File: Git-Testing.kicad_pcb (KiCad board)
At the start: 2 copper layers, 6 parts, among them J1 Conn_01x02_Male, J2 Conn_01x02_Male

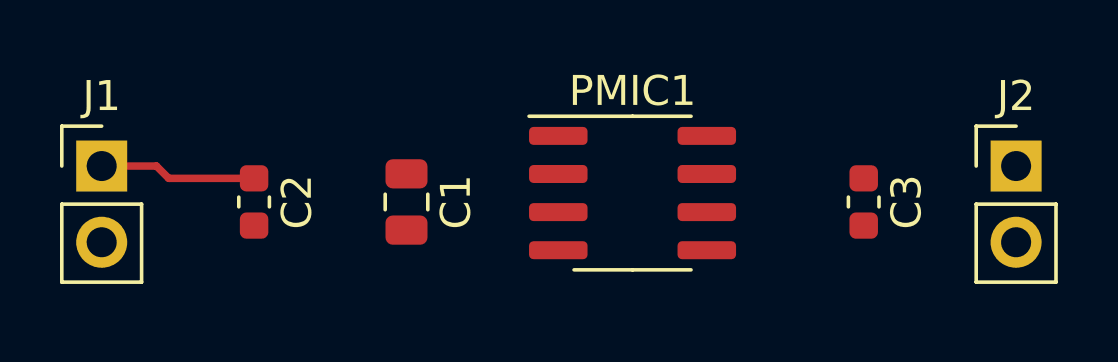
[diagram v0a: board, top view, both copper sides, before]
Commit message: Se termino la pcb
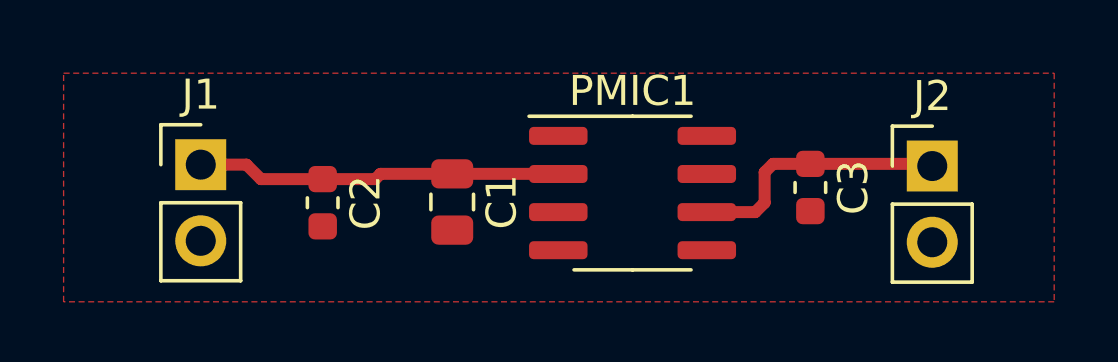
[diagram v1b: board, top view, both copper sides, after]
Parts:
- moved J1 3.30 mm to (118.9, 102.1)
- moved J2 2.79 mm to (143.3, 102.2)
- moved C2 2.29 mm to (122.9, 103.4)
- moved C3 1.84 mm to (139.2, 102.9)
- moved C1 1.52 mm to (127.3, 103.4)
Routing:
- net Net-(C3-Pad1): track 0.00 -> 8.81 mm
- net VCC: track 5.25 -> 12.2 mm
- added copper zone on F.Cu, net GND
